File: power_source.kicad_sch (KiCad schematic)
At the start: 19 parts, among them J2 USB_B_Micro, Q1 Q_PMOS_GDS, Q2 BSS138, SW2 SW_SPDT

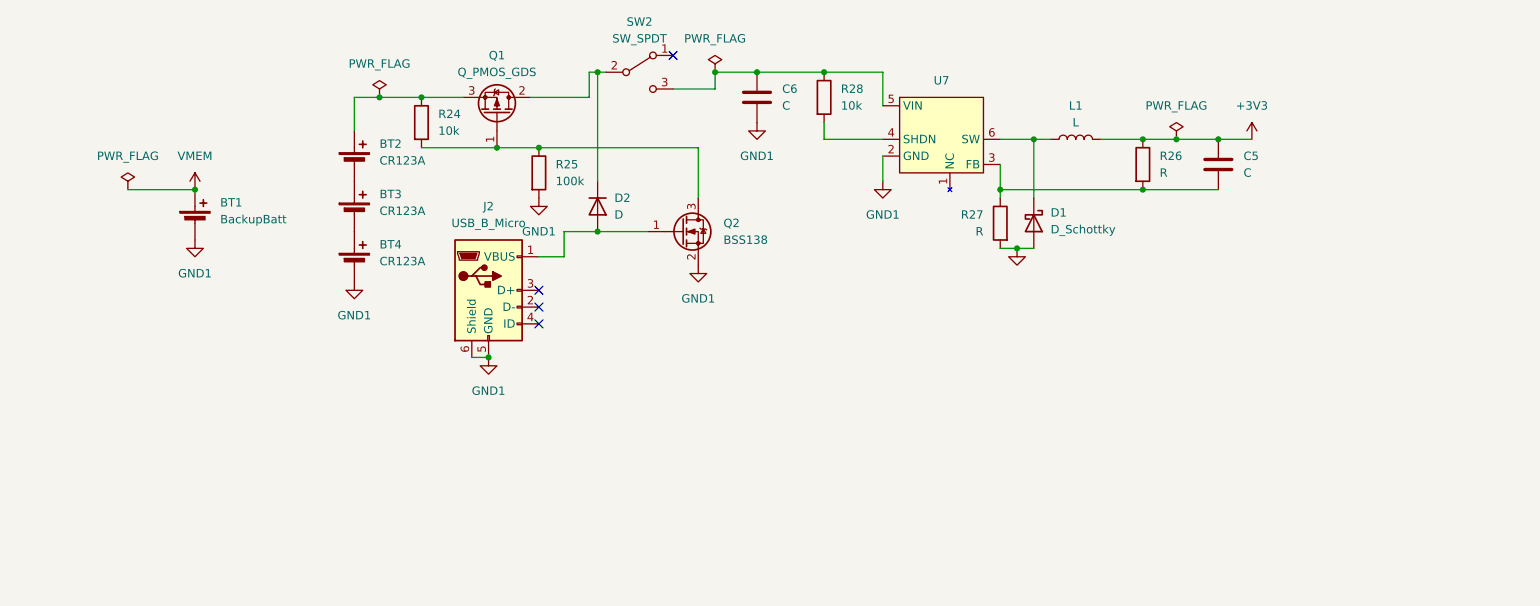
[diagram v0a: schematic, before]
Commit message: make board
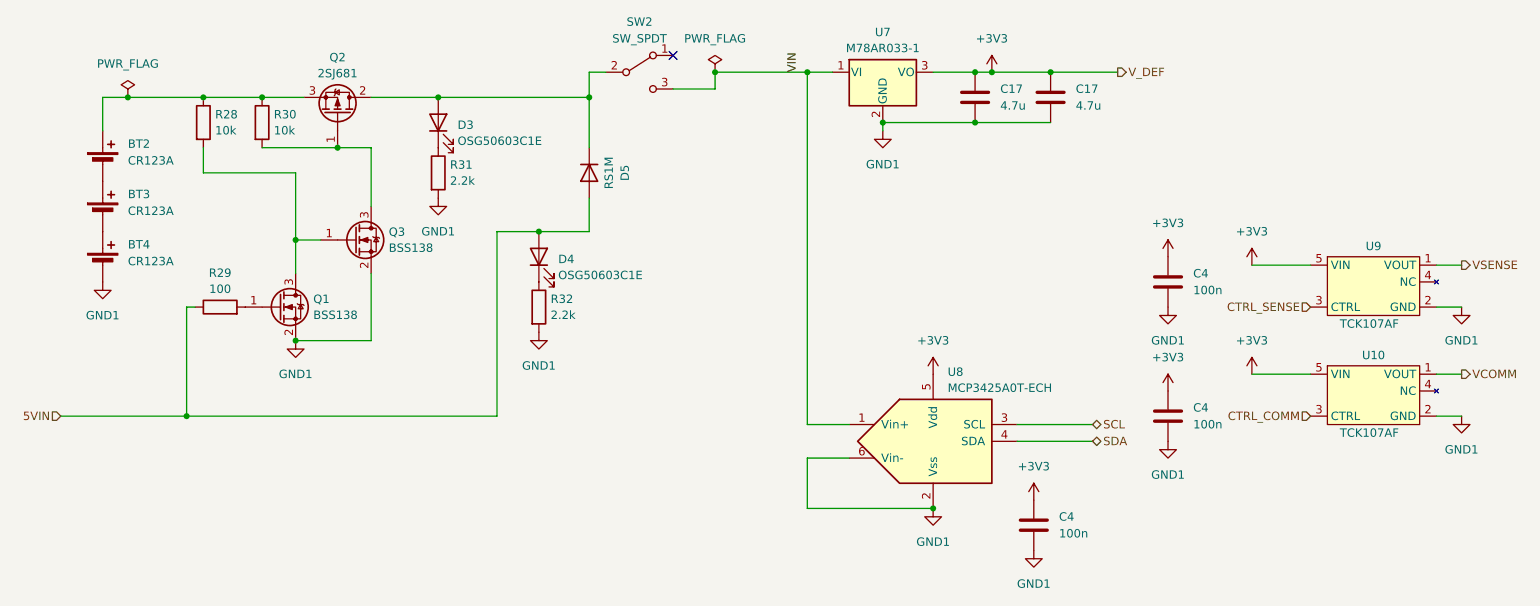
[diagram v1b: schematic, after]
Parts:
- removed BT1: BackupBatt, symbol Device:Battery_Cell
- removed C5, C6: C, symbol Device:C
- removed D1: D_Schottky, symbol Device:D_Schottky
- removed D2: D, symbol Device:D
- removed J2: USB_B_Micro, symbol Connector:USB_B_Micro
- removed L1: L, symbol Device:L
- removed Q1: Q_PMOS_GDS, symbol Device:Q_PMOS_GDS
- removed Q2: BSS138, Package_TO_SOT_SMD:SOT-23, symbol Transistor_FET:BSS138
- removed R24: 10k, symbol Device:R
- removed R25: 100k, symbol Device:R
- removed R26, R27: R, symbol Device:R
- removed U7: ~, symbol balloon_lib:NJW1616F1-AT
- added C17 (x2): 4.7u, Capacitor_SMD:C_0603_1608Metric_Pad1.08x0.95mm_HandSolder, symbol Device:C
- added C4 (x3): 100n, Capacitor_SMD:C_0603_1608Metric_Pad1.08x0.95mm_HandSolder, symbol Device:C
- added D3, D4: OSG50603C1E, LED_SMD:LED_0603_1608Metric_Pad1.05x0.95mm_HandSolder, symbol Device:LED
- added D5: RS1M, Diode_SMD:D_SMA_Handsoldering, symbol Device:D
- added Q1, Q3: BSS138, Package_TO_SOT_SMD:SOT-23, symbol Transistor_FET:BSS138
- added Q2: 2SJ681, Package_TO_SOT_THT:SIPAK_Vertical, symbol Device:Q_PMOS_GDS
- added R29: 100, Resistor_SMD:R_0603_1608Metric_Pad0.98x0.95mm_HandSolder, symbol Device:R
- added R30: 10k, Resistor_SMD:R_0603_1608Metric_Pad0.98x0.95mm_HandSolder, symbol Device:R
- added R31, R32: 2.2k, Resistor_SMD:R_0603_1608Metric_Pad0.98x0.95mm_HandSolder, symbol Device:R
- added U10, U9: TCK107AF, Package_TO_SOT_SMD:SOT-23-5_HandSoldering, symbol balloon_lib:TCK107
- added U7: M78AR033-1, Package_TO_SOT_THT:TO-220-3_Vertical, symbol Regulator_Linear:LM7805_TO220
- added U8: MCP3425A0T-ECH, Package_TO_SOT_SMD:SOT-23-6_Handsoldering, symbol Analog_ADC:MCP3425A0T-ECH
- BT2, BT3, BT4: footprint (none) -> balloon:CR123A
- R28: footprint (none) -> Resistor_SMD:R_0603_1608Metric_Pad0.98x0.95mm_HandSolder
- SW2: footprint (none) -> Connector_PinSocket_2.54mm:PinSocket_1x03_P2.54mm_Vertical
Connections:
- net +3V3: now also C17.1, C17.1, C4.1, C4.1, C4.1, U10.5 (VIN), U7.3 (VO), U8.5 (Vdd), U9.5 (VIN)
- net GND1: now also C17.2, C17.2, C4.2, C4.2, C4.2, Q1.2 (S), Q3.2 (S), R31.2, R32.2, U10.2 (GND), U7.2 (GND), U8.2 (Vss), U8.6 (Vin-), U9.2 (GND)
- net at R28.1: now also BT2.1 (+), Q2.3 (S), R30.1; no longer SW2.3 (C)
- net at R28.2: now also Q1.3 (D), Q3.1 (G)
- net at SW2.2 (B): now also D3.2 (A), D5.1 (K), Q2.2 (D)
- new net: D4.1 (K), R32.1
- new net: Q2.1 (G), Q3.3 (D), R30.2
- new net: D3.1 (K), R31.1
- new net: Q1.1 (G), R29.2
- new net 5VIN: D4.2 (A), D5.2 (A), R29.1
- new net CTRL_COMM: U10.3 (CTRL)
- new net CTRL_SENSE: U9.3 (CTRL)
- new net SCL: U8.3 (SCL)
- new net SDA: U8.4 (SDA)
- new net VCOMM: U10.1 (VOUT)
- new net VIN: SW2.3 (C), U7.1 (VI), U8.1 (Vin+)
- new net VSENSE: U9.1 (VOUT)
- no-connect marks 4 -> 1
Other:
- moved on the sheet: BT2, BT3, BT4
